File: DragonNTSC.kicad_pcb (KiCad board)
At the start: 2 copper layers, 120.2 x 35.7 mm, 19 parts, among them IC1 74LS273N, IC2 MC6847, IC3 MC1372, J1 Video Output, J2 Board Interconnect Male, Q1 2N4403, Q2 2N4401

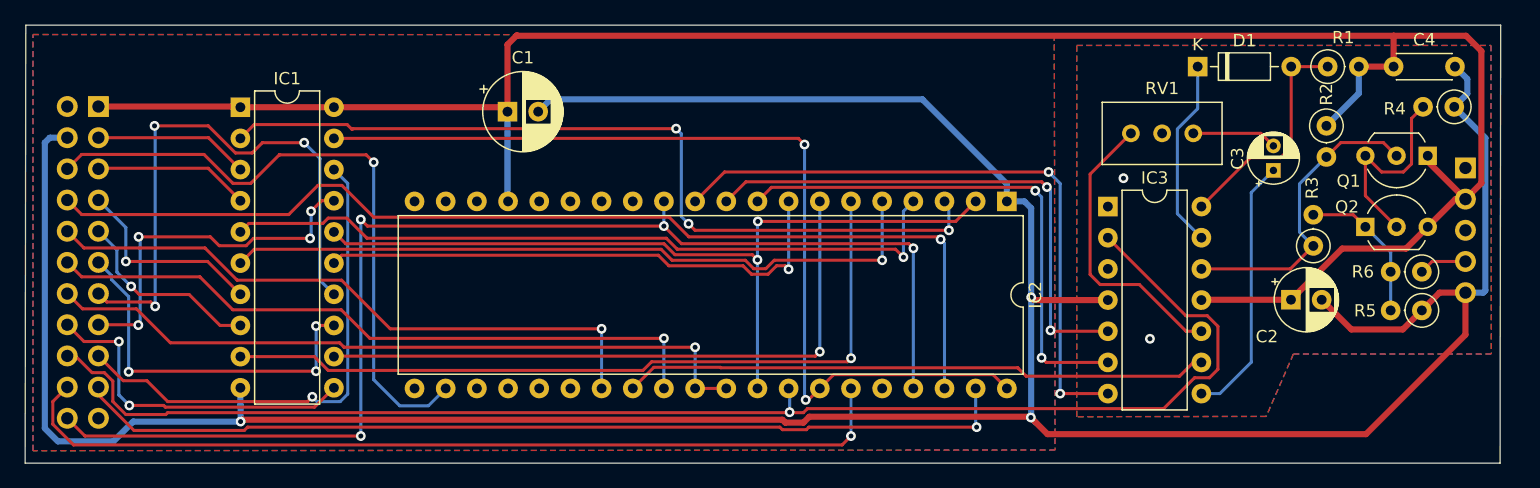
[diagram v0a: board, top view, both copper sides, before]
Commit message: prepare alpha2 build
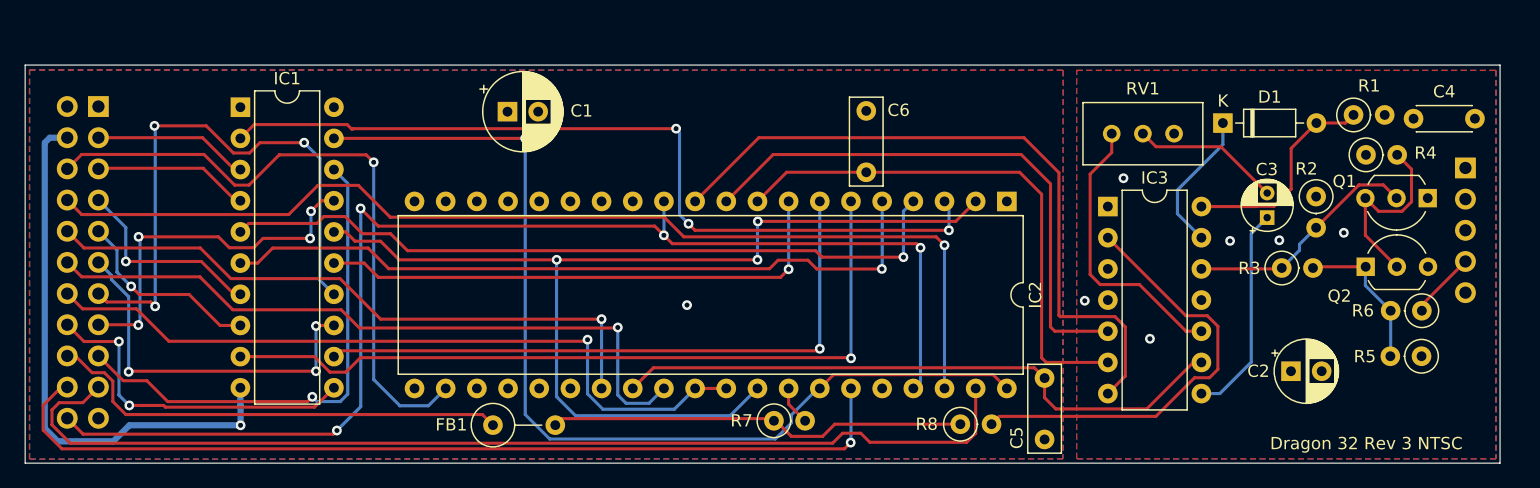
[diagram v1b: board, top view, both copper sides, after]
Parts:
- added C5: 150pF, Capacitor_THT:C_Rect_L7.0mm_W2.5mm_P5.00mm, F.Cu at (164.4, 130.8)
- added C6: 0.1uF, Capacitor_THT:C_Rect_L7.0mm_W2.5mm_P5.00mm, F.Cu at (149.9, 104.0)
- added FB1: ?uH, Inductor_THT:L_Axial_L7.0mm_D3.3mm_P5.08mm_Vertical_Fastron_MICC, F.Cu at (119.4, 129.6)
- added R7: 150R, Resistor_THT:R_Axial_DIN0207_L6.3mm_D2.5mm_P2.54mm_Vertical, F.Cu at (142.3, 129.2)
- added R8: 10k, Resistor_THT:R_Axial_DIN0207_L6.3mm_D2.5mm_P2.54mm_Vertical, F.Cu at (157.5, 129.5)
- moved R4 8.19 mm to (190.6, 107.6), turned to 0 degrees
- moved R2 5.83 mm to (186.5, 111.0)
- moved C2 5.82 mm to (184.5, 125.2)
- moved D1 5.04 mm to (178.9, 105.0)
- moved C4 4.54 mm to (194.5, 104.6)
- moved R1 4.47 mm to (189.6, 104.3)
- moved C3 3.88 mm to (182.5, 112.7)
- moved R5 3.73 mm to (195.1, 124.0)
- moved Q1 3.45 mm to (195.6, 111.1)
- moved Q2 3.25 mm to (190.6, 116.7)
- moved R6 3.18 mm to (195.1, 120.3)
- moved R3 3.14 mm to (183.7, 116.8), turned to 0 degrees
- moved RV1 1.57 mm to (174.9, 105.8)
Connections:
- net Net-(IC1-Q0) renamed /D0
- net Net-(IC1-Q1) renamed /D1
- net Net-(IC1-Q2) renamed /D2
- net Net-(IC1-Q3) renamed /D3
- net Net-(IC1-Q4) renamed /D4
- net Net-(IC1-Q5) renamed /D5
- net Net-(IC1-Q6) renamed /D6
- net Net-(IC1-Q7) renamed /D7
- IC2 pad 33: VCLK -> Net-(IC2-CLK)
- IC3 pad 2: VCLK -> Net-(IC3-OSC)
- J2 pad 18: VCLK -> Net-(J2-Pin_18)
- RV1 pad 1: Net-(C3-Pad2) -> unconnected-(RV1-Pad1)
- RV1 pad 2: unconnected-(RV1-Pad2) -> Net-(C3-Pad2)
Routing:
- net GND: track 258.1 -> 45.5 mm, vias 5 -> 8
- net +5V: track 180.1 -> 0.00 mm
- net VCLK: track 115.7 -> 34.2 mm, vias 1 -> 0
- net Net-(J2-Pin_18): track 0.00 -> 38.0 mm
- net Net-(IC3-OSC): track 0.00 -> 35.8 mm
- net /D6: track 67.5 -> 86.1 mm, vias 2 -> 3
- net CSS: track 76.9 -> 86.2 mm, vias 1 -> 0
- net Composite: track 25.2 -> 19.5 mm
- net Net-(C3-Pad2): track 6.95 -> 12.1 mm
- net phiA: track 52.1 -> 56.4 mm, vias 2 -> 0
- net /D7: track 77.1 -> 81.2 mm, vias 2 -> 1
- net Net-(IC3-ChrMod): track 21.5 -> 17.4 mm
- net Net-(D1-K): track 15.4 -> 11.7 mm
- net Net-(IC2-CLK): track 0.00 -> 3.19 mm
- net LUM: track 47.8 -> 50.9 mm
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- added copper zone on In2.Cu, net +5V
- added copper zone on In1.Cu, net GND
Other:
- board size 120.2 x 35.7 mm -> 120.2 x 32.4 mm
- copper layers 2 -> 4
- board text added: "Dragon 32 Rev 3 NTSC"
